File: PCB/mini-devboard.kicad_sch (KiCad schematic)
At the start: 16 parts, among them J1 USB_A, J2 Conn_02x05_Counter_Clockwise, SW1 SW_Push, U1 CH552G

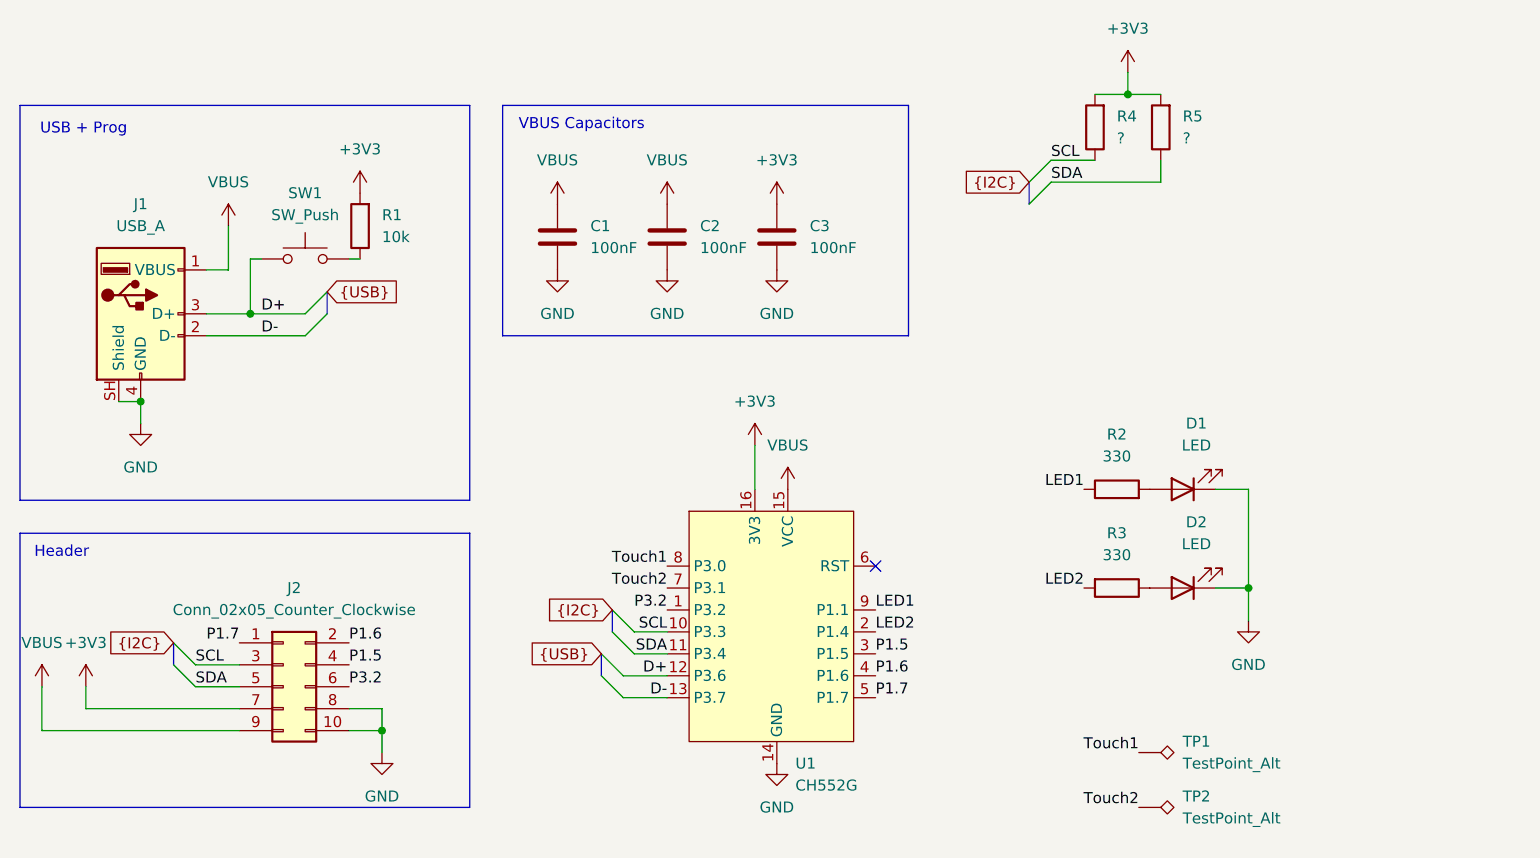
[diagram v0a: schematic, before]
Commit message: organization
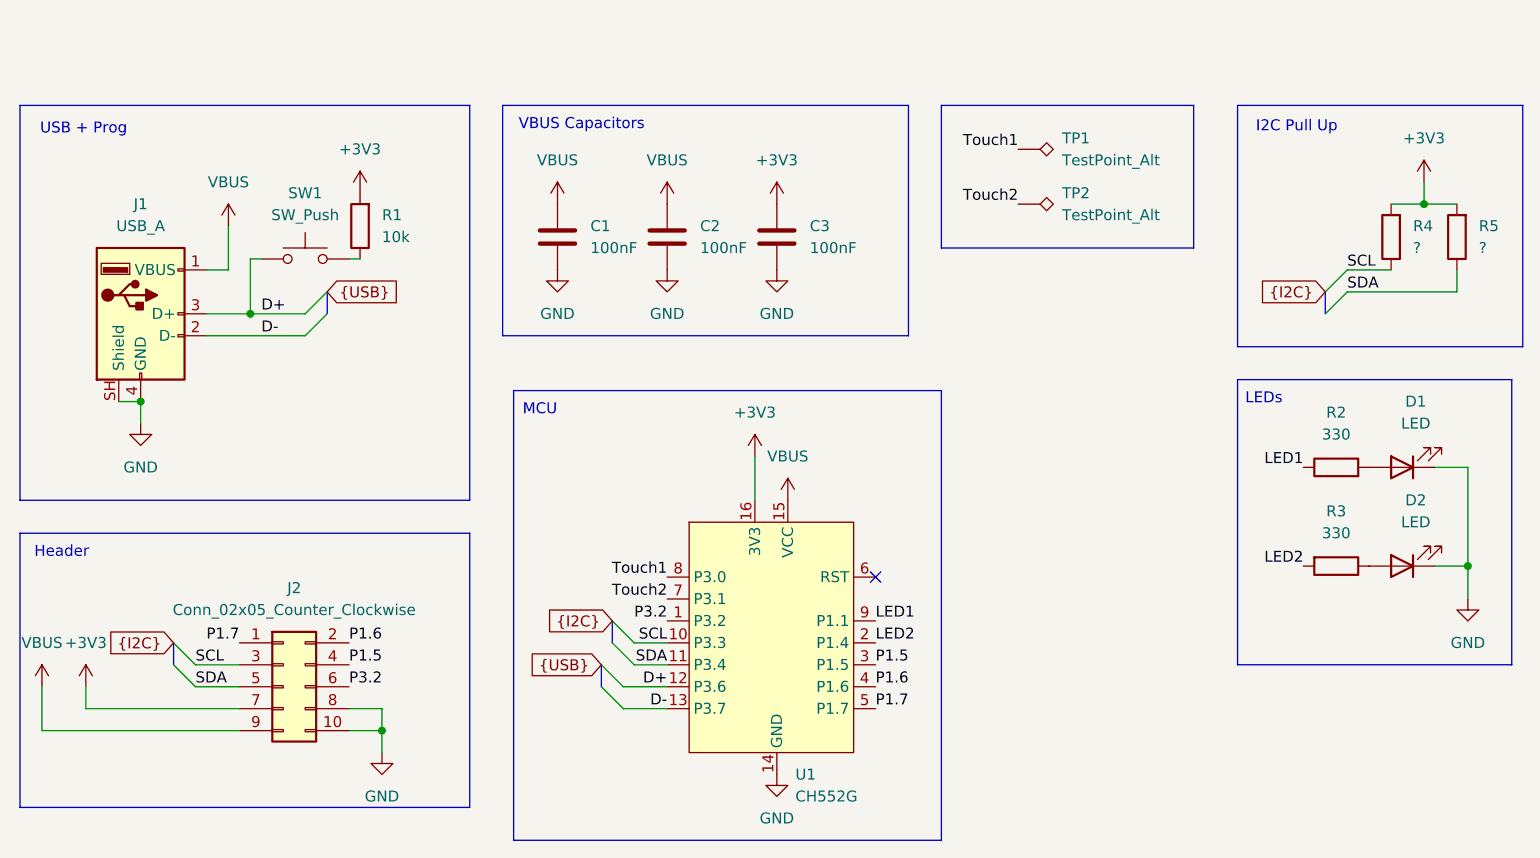
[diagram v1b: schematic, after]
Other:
- note added: "I2C Pull Up"
- note added: "LEDs"
- note added: "MCU"
- moved on the sheet: D1, D2, R2, R3, R4, R5, TP1, TP2, U1
